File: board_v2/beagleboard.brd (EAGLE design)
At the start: 69.8 x 54.6 mm, 40 parts, among them U1 DWM1000, X1 5566-2, X2 04-JST-B4B-XH-A

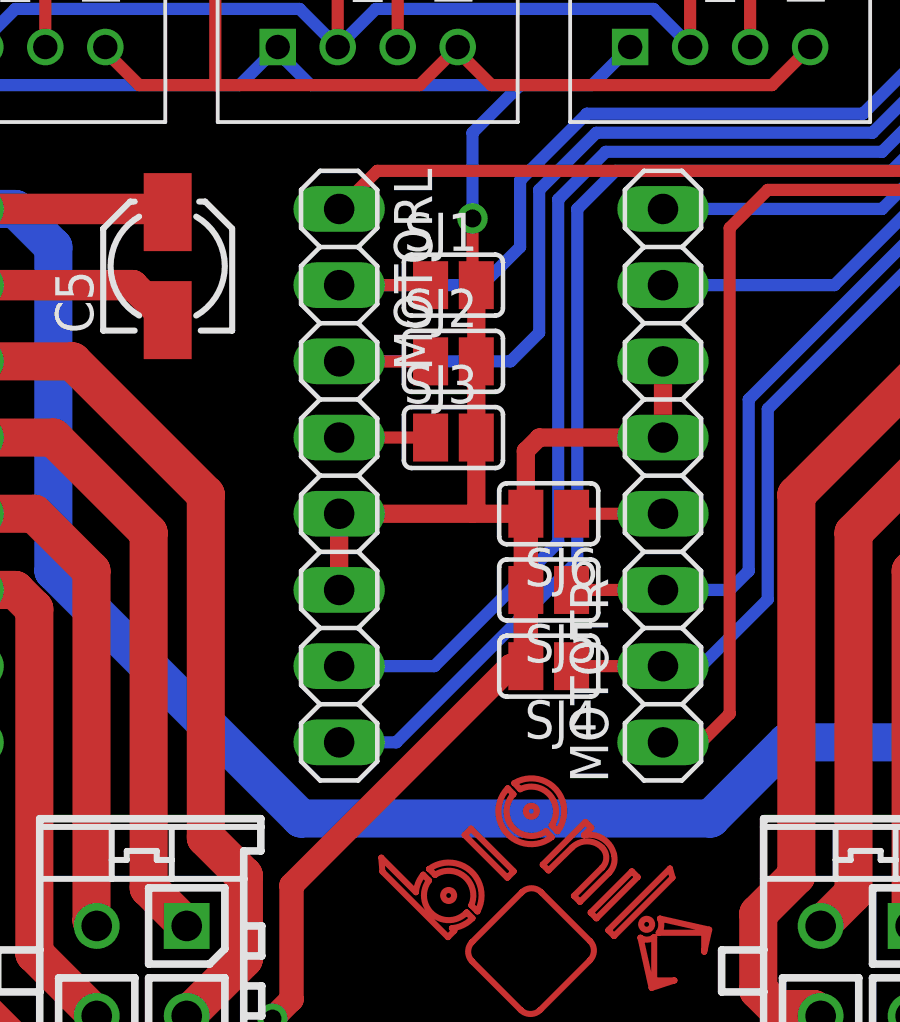
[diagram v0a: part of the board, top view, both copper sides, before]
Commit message: pullups
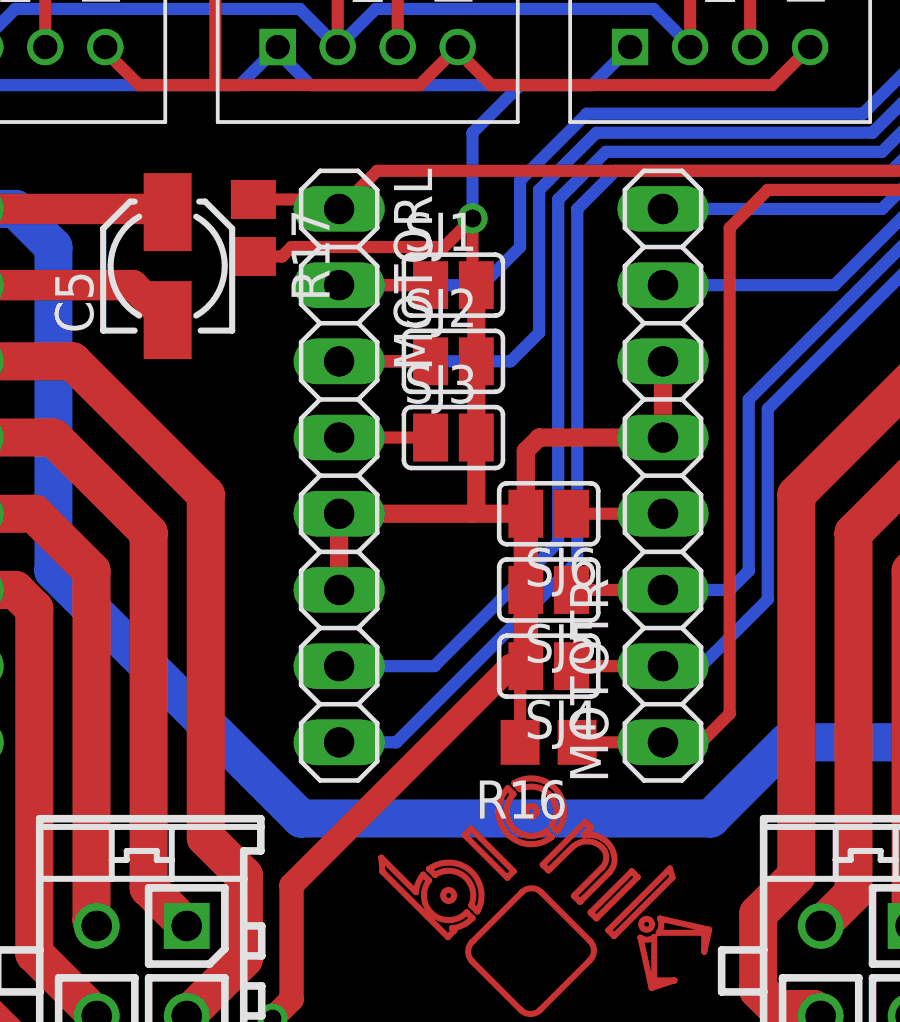
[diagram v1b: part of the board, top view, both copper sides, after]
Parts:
- added R16, R17: 10k, rcl:R0805
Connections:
- net +5V: now also R16.2, R17.2
- net MLEN: now also R17.1
- net MREN: now also R16.1
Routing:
- net +5V: track 174.5 -> 185.0 mm
- net MLEN: track 40.1 -> 43.1 mm
- net MREN: track 44.2 -> 47.0 mm
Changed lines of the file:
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@@
 <element name="R14" library="rcl" package="R0805" value="" x="33.02" y="46.99" rot="R270"/>
 <element name="R15" library="rcl" package="R0805" value="" x="31.115" y="46.99" rot="R90"/>
+<element name="R16" library="rcl" package="R0805" value="10k" x="26.3525" y="20.0025" rot="R180"/>
+<element name="R17" library="rcl" package="R0805" value="10k" x="16.51" y="37.1475" rot="R270"/>
 </elements>
 <signals>
@@
 <wire x1="17.145" y1="10.4775" x2="12.7" y2="6.0325" width="0.8128" layer="16"/>
 <wire x1="12.7" y1="6.0325" x2="12.7" y2="5.08" width="0.8128" layer="16"/>
+<contactref element="R16" pad="2"/>
+<contactref element="R17" pad="2"/>
+<wire x1="16.51" y1="36.1975" x2="17.465" y2="36.1975" width="0.4064" layer="1"/>
+<wire x1="17.465" y1="36.1975" x2="17.78" y2="36.5125" width="0.4064" layer="1"/>
+<wire x1="17.78" y1="36.5125" x2="22.86" y2="36.5125" width="0.4064" layer="1"/>
+<wire x1="22.86" y1="36.5125" x2="23.8125" y2="37.465" width="0.4064" layer="1"/>
+<wire x1="25.4025" y1="20.0025" x2="25.4025" y2="22.3545" width="0.4064" layer="1"/>
+<wire x1="25.4025" y1="22.3545" x2="25.5905" y2="22.5425" width="0.4064" layer="1"/>
 </signal>
 <signal name="CSN">
@@
 <wire x1="40.3225" y1="39.0525" x2="20.6375" y2="39.0525" width="0.4064" layer="1"/>
 <wire x1="20.6375" y1="39.0525" x2="19.3675" y2="37.7825" width="0.4064" layer="1"/>
+<contactref element="R17" pad="1"/>
+<wire x1="16.51" y1="38.0975" x2="19.0525" y2="38.0975" width="0.4064" layer="1"/>
+<wire x1="19.0525" y1="38.0975" x2="19.3675" y2="37.7825" width="0.4064" layer="1"/>
 </signal>
 <signal name="MOSI">
@@
 <wire x1="32.385" y1="20.955" x2="31.4325" y2="20.0025" width="0.4064" layer="1"/>
 <wire x1="31.4325" y1="20.0025" x2="30.1625" y2="20.0025" width="0.4064" layer="1"/>
+<contactref element="R16" pad="1"/>
+<wire x1="27.3025" y1="20.0025" x2="30.1625" y2="20.0025" width="0.4064" layer="1"/>
 </signal>
 <signal name="DWMRES">
